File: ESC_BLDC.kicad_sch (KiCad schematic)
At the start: 95 parts, among them J1 Conn_01x06_Pin, J2 Conn_01x04_Pin, U4 LM339, U5 AP1509-50SG-13, U6 MCP6002-xP, U7 MCP6002-xP, U8 MCP6002-xP

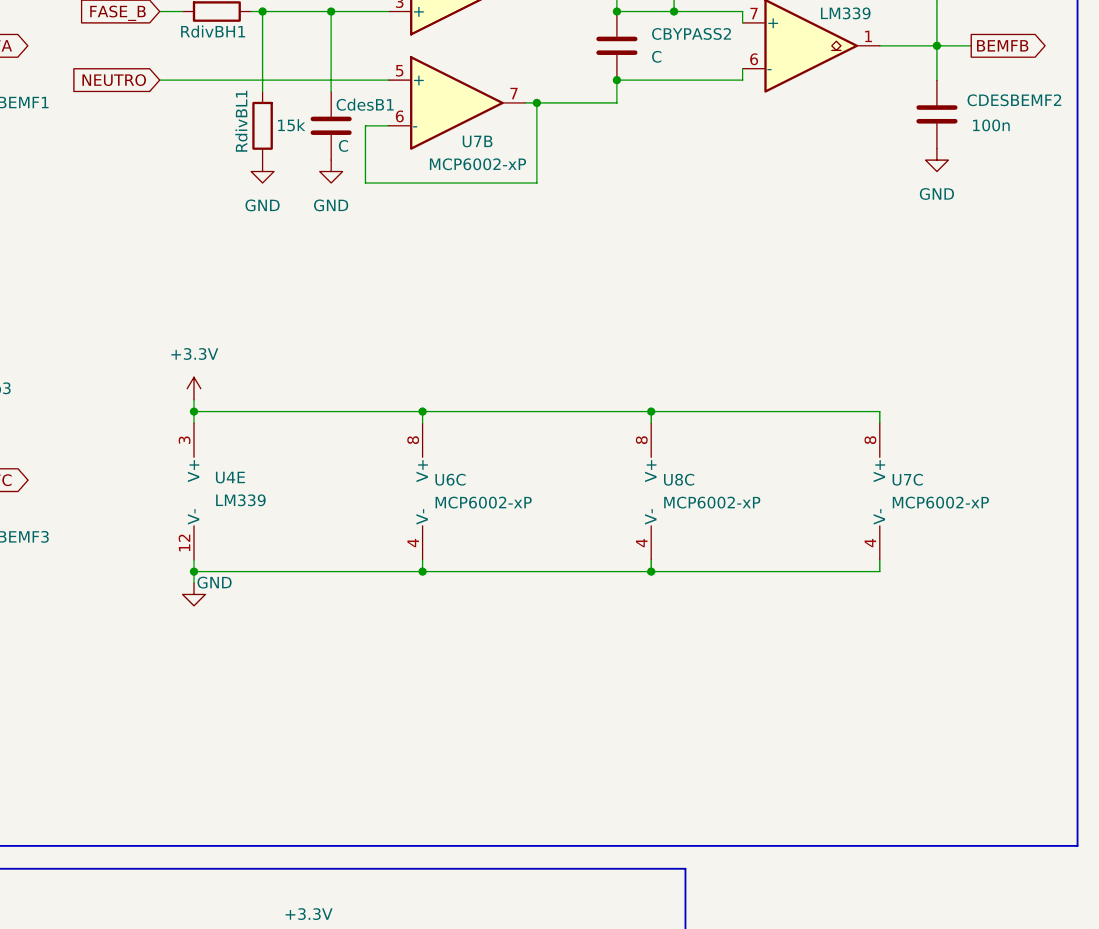
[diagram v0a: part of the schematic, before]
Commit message: ordenado por funcion
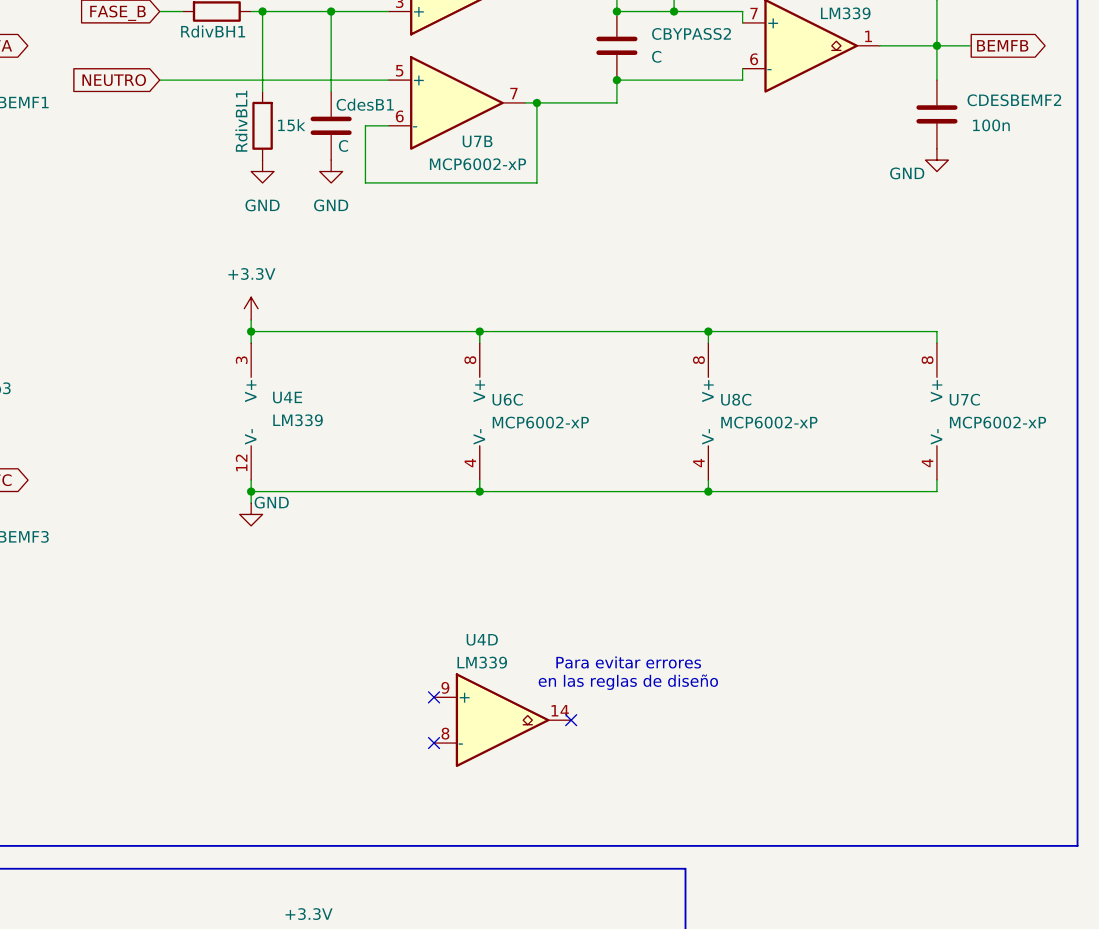
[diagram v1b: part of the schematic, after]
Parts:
- added unit 4 of U4
- DBUCK1: footprint Diode_SMD:D_1206_3216Metric_Pad1.42x1.75mm_HandSolder -> Diode_THT:D_DO-34_SOD68_P7.62mm_Horizontal
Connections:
- no-connect marks 28 -> 31
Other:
- note added: "Para evitar errores en las reglas de diseño"
- moved on the sheet: U4E, U6C, U7C, U8C
